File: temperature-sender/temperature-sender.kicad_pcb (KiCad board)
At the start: 2 copper layers, 50 x 25 mm, 46 parts, among them IC1 ATTINY2313A-S, K1 SERVO, P1 ISP, P2 CONN_01X02, P3 CONN_01X03, P4 CONN_01X04, P5 CONN_01X03, P6 03mmTo05mm, P7 03mmTo05mm, SW1 SW_PUSH, SW2 SW_PUSH, U1 AMS1117, U2 LM317L, U3 TMP102

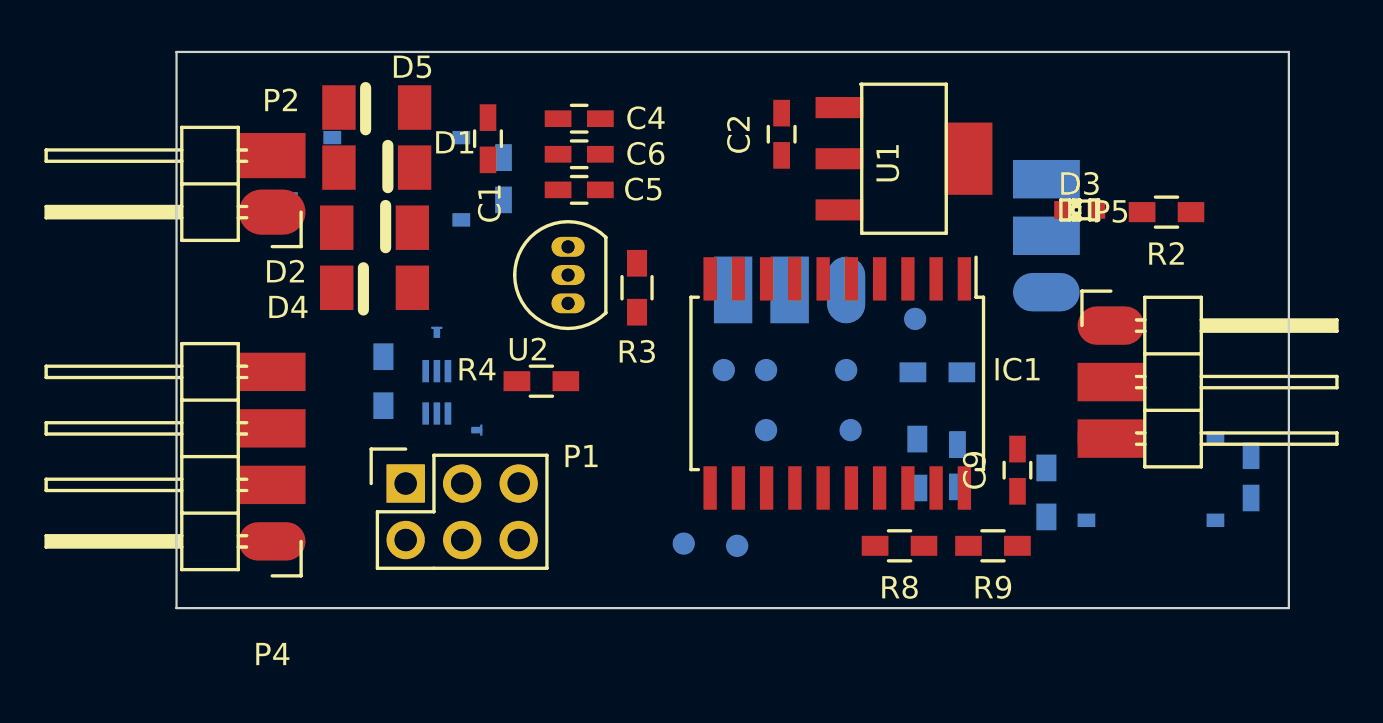
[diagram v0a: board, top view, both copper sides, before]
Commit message: Temperature sender before import freerouting results
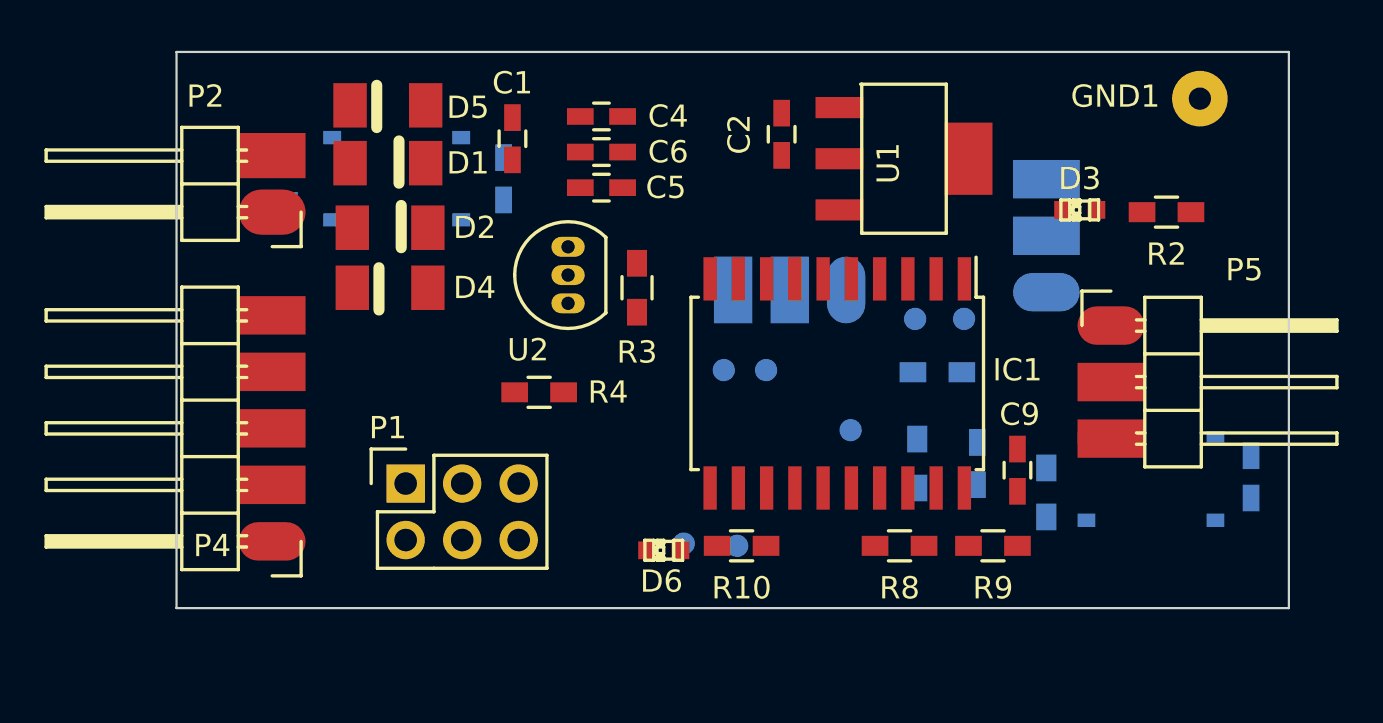
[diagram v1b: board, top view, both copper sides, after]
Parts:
- removed P6, P7: 03mmTo05mm, kicad-footprints:03mmTo05mm
- removed TP_PB2: TEST_POINT, kicad-footprints:TP_1mm
- removed U3: TMP102, kicad-footprints:SOT563
- added D6: Led_Small, LEDs:LED-0603, F.Cu at (126.9, 142.4)
- added GND1: TEST_POINT, Wire_Pads:SolderWirePad_single_1mmDrill, F.Cu at (151.0, 122.1)
- P4: value CONN_01X04 -> CONN_01X05; footprint kicad-footprints:Pin_Header_Angled_SMD_1x04 -> kicad-footprints:Pin_Header_Angled_SMD_1x05
- R10: value 5k -> 330R; moved to F.Cu
- moved R10 17.7 mm to (130.4, 142.2), turned to 180 degrees
- moved TP_XTAL2 5.78 mm to (140.3, 132.0)
- moved C1 1.10 mm to (120.1, 123.9)
- moved C5 1.00 mm to (124.1, 126.1)
- moved C4 1.00 mm to (124.1, 122.9)
- moved C6 1.00 mm to (124.1, 124.5)
- moved C8 0.91 mm to (141.0, 138.5)
- moved D2 0.70 mm to (114.6, 127.9)
- moved D4 0.70 mm to (114.6, 130.6)
- moved D1 0.54 mm to (114.5, 125.0)
- moved R4 0.51 mm to (121.3, 135.3)
- moved D5 0.51 mm to (114.5, 122.4)
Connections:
- R10 pad 1: /ALERT -> Net-(IC1-Pad13)
- R10 pad 2: /03mm3.3V -> Net-(D6-Pad2)
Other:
- net class 3V3: trace_width 0.25 -> 0.5
- net class GND: trace_width 0.25 -> 0.5

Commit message: Unknown changes, probably what I ordered
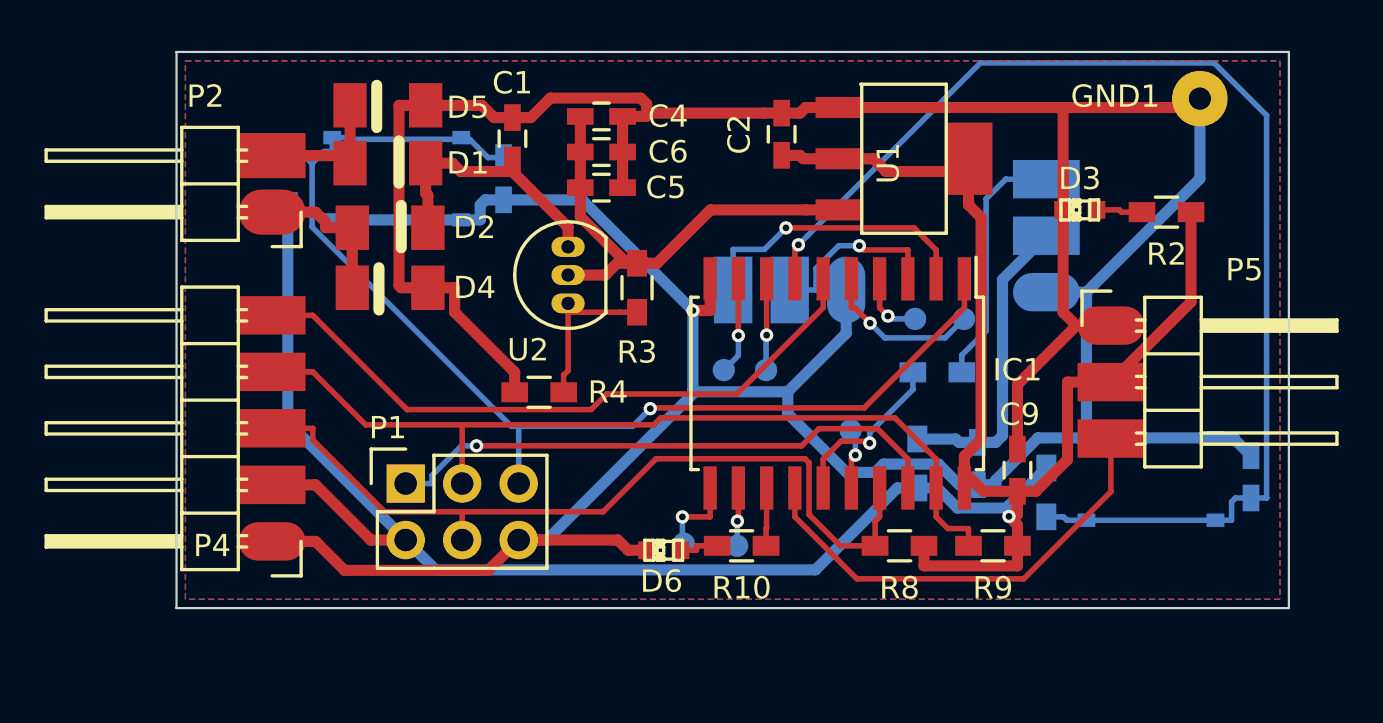
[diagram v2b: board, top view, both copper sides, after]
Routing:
- net GND: track 0.00 -> 184.1 mm, vias 0 -> 1
- net +3V3: track 0.00 -> 109.8 mm, vias 0 -> 1
- net /SW: track 0.00 -> 55.1 mm, vias 0 -> 1
- net /RESET: track 0.00 -> 53.1 mm, vias 0 -> 1
- net /SCL: track 0.00 -> 39.4 mm
- net /SDA/MOSI: track 0.00 -> 36.9 mm
- net /ALERT: track 0.00 -> 29.7 mm
- net /MISO: track 0.00 -> 25.7 mm, vias 0 -> 1
- net /9v: track 0.00 -> 20.9 mm
- net /RF_DATA: track 0.00 -> 20.7 mm
- net /SERVO_PWR: track 0.00 -> 13.8 mm
- net /RX: track 0.00 -> 13.1 mm, vias 0 -> 1
- net /Vin_rec: track 0.00 -> 12.0 mm
- net /SERVO_SIG: track 0.00 -> 11.3 mm
- net /TX: track 0.00 -> 8.09 mm, vias 0 -> 1
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- added copper zone on F.Cu, net +3V3
- added copper zone on B.Cu, net GND
